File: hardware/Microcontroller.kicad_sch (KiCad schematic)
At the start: 10 parts

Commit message: added mouser part numbers
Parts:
- A1, R3, R4, R46, R47, R48, R49, R5, R58, R6: Part Source (none) -> Uni

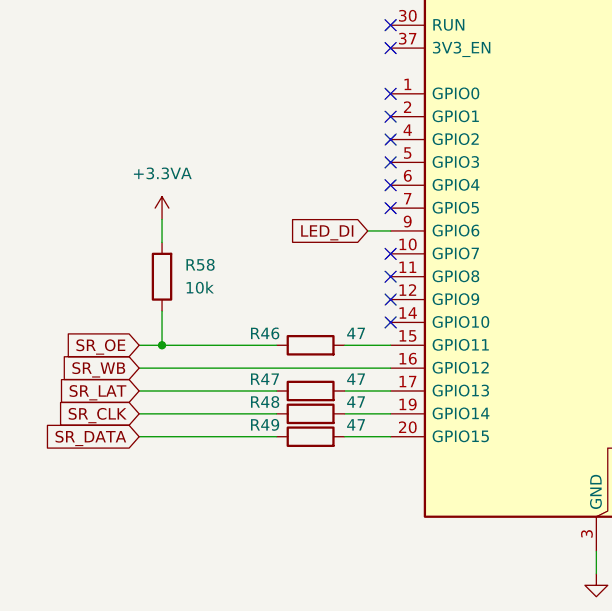
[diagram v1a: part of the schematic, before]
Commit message: more routing progress
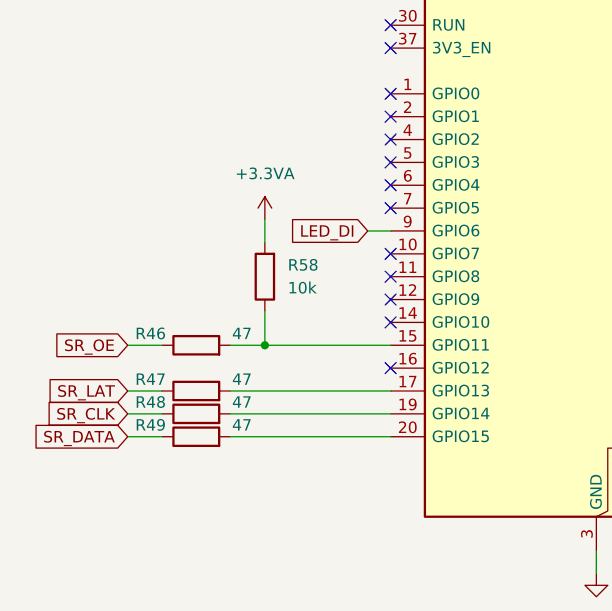
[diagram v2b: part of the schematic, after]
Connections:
- net SR_OE: no longer R58.1
- net at A1.15 (GPIO11), R46.2: now also R58.1
- net SR_WB: no longer names the net of A1.16 (GPIO12)
- no-connect marks 19 -> 20
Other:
- moved on the sheet: R46, R47, R48, R49
